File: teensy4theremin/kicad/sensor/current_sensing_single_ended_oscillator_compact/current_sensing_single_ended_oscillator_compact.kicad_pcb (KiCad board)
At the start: 2 copper layers, 70.5 x 21.1 mm, 25 parts, among them J1 ANTENNA, J2 INDUCTOR_OUT, J3 INDUCTOR_IN, J6 OSC, U1 4220CZ6, U2 LD3985M33R_SOT23, U3 LT1711xMS8

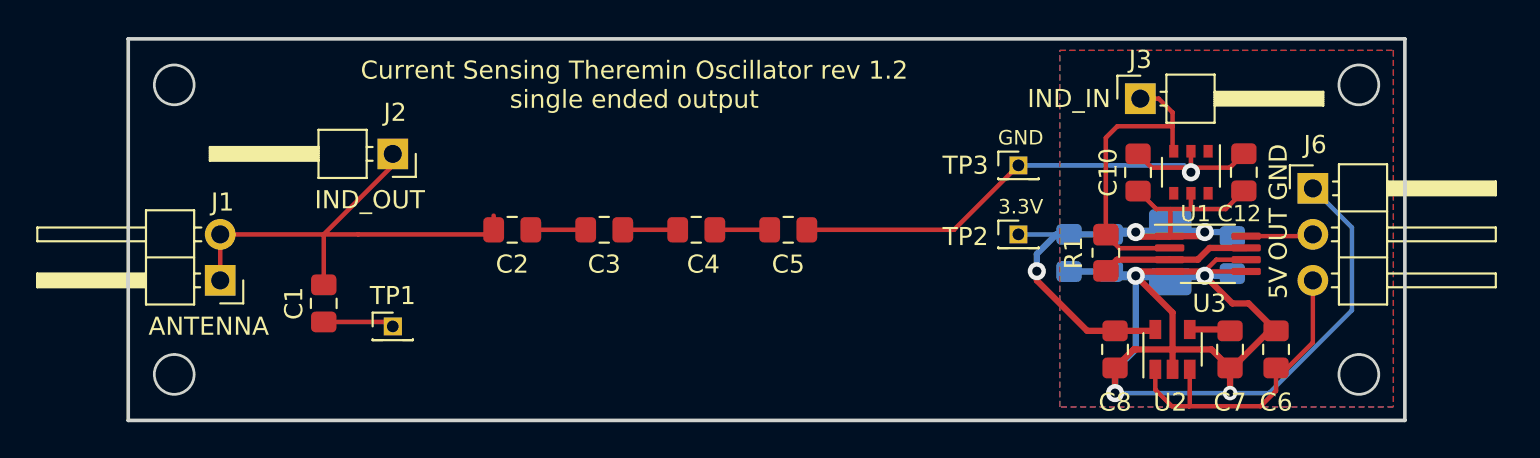
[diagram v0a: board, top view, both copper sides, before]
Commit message: update sensor
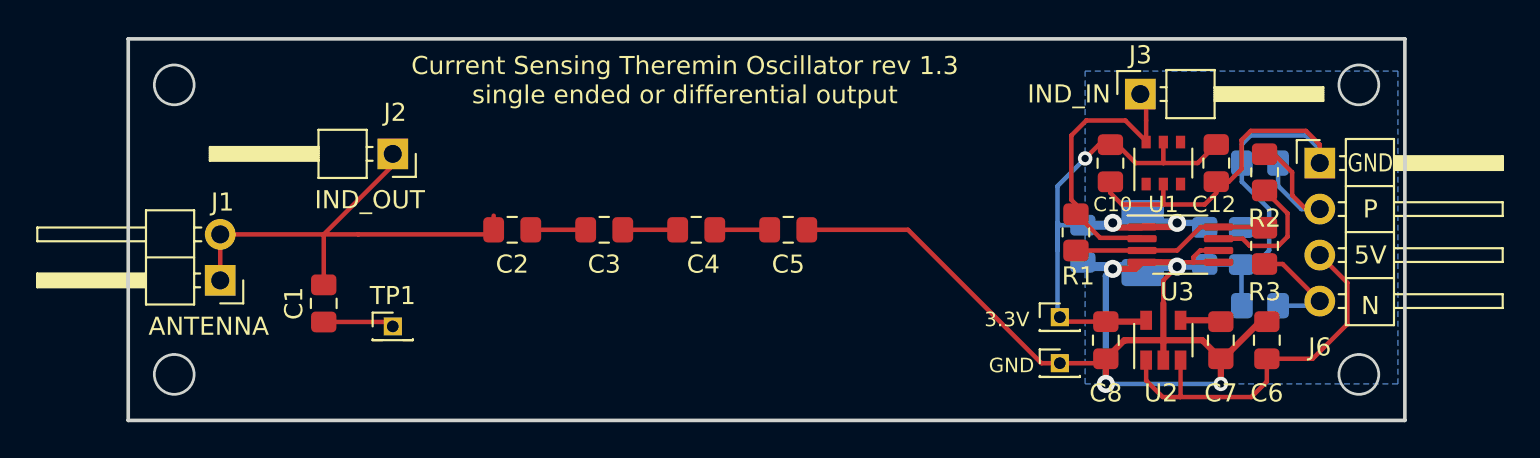
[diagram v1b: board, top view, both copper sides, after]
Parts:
- added R2: 10, Resistor_SMD:R_0805_2012Metric_Pad1.20x1.40mm_HandSolder, F.Cu at (144.0, 101.3)
- added R3: 10, Resistor_SMD:R_0805_2012Metric_Pad1.20x1.40mm_HandSolder, F.Cu at (144.0, 105.4)
- added R4: 100, Resistor_SMD:R_0805_2012Metric_Pad1.20x1.40mm_HandSolder, B.Cu at (143.8, 108.7)
- added R5: 100, Resistor_SMD:R_0805_2012Metric_Pad1.20x1.40mm_HandSolder, B.Cu at (143.8, 100.8)
- C12, C8: value 1uF -> 2.2uF
- J6: footprint Connector_PinHeader_2.54mm:PinHeader_1x03_P2.54mm_Horizontal -> Connector_PinHeader_2.54mm:PinHeader_1x04_P2.54mm_Horizontal
- U2: value LD3985M33R_SOT23 -> LP2985AIM5-3.3
- U3: value LT1711xMS8 -> LT1711CMS8
- moved TP3 11.2 mm to (132.7, 111.9)
- moved C14 9.53 mm to (142.7, 105.4)
- moved TP2 5.11 mm to (132.7, 109.3)
- moved R1 2.00 mm to (133.6, 104.7)
- moved C10 1.61 mm to (135.5, 100.8), turned to 270 degrees
- moved C12 1.61 mm to (141.4, 100.8), turned to 270 degrees
- moved C13 1.61 mm to (140.7, 105.4)
- moved U1 1.61 mm to (138.4, 100.8), turned to 90 degrees
- moved C11 1.61 mm to (137.3, 105.3)
- moved U3 1.61 mm to (139.4, 105.3)
- moved C9 1.61 mm to (134.0, 105.3)
- moved J6 1.45 mm to (147.1, 100.8)
- moved C7 0.72 mm to (141.6, 110.6)
- moved C8 0.72 mm to (135.3, 110.6)
- moved C6 0.72 mm to (144.1, 110.6)
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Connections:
- J3 pad 1: Net-(J3-Pad1) -> /IND_IN
- J6 pad 2: /OUT_P -> /OUTP
- R1 pad 1: Net-(R1-Pad1) -> /DRIVE
- R1 pad 2: Net-(J3-Pad1) -> /IND_IN
- U1 pad 3: Net-(J3-Pad1) -> Net-(U1-Pad3)
- U1 pad 6: Net-(U1-Pad6) -> /IND_IN
- U3 pad 2: Net-(J3-Pad1) -> /IND_IN
- U3 pad 3: Net-(R1-Pad1) -> /DRIVE
- U3 pad 7: Net-(R1-Pad1) -> Net-(R2-Pad1)
- U3 pad 8: /OUT_P -> /DRIVE
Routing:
- net Net-(J3-Pad1): track 17.4 -> 0.00 mm
- net /IND_IN: track 0.00 -> 16.4 mm
- net /DRIVE: track 0.00 -> 11.0 mm
- net /OUTP: track 0.00 -> 9.14 mm
- net Net-(R1-Pad1): track 8.27 -> 0.00 mm
- net Net-(R2-Pad1): track 0.00 -> 7.27 mm
- net /OUTN: track 0.00 -> 6.30 mm
- net /OUT_P: track 3.72 -> 0.00 mm
- net /5V: track 17.9 -> 21.5 mm
- net /3V3_A: track 37.6 -> 40.9 mm
- net GND: track 105.0 -> 104.8 mm, vias 5 -> 4
- removed copper zone on F.Cu, net GND
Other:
- board text added: "+5V"
- board text added: "Current Sensing Theremin Oscillator rev 1.3 single ended or differential output"
- board text added: "N"
- board text added: "OUTN"
- board text added: "OUTP"
- board text added: "P"
- board text removed: "Current Sensing Theremin Oscillator rev 1.2 single ended output"
- board text removed: "OUT"
- board text removed: "V_IN"
